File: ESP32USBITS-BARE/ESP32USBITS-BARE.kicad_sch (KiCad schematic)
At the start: 45 parts, among them IC2 74LVC, IC3 5PB1102, IC4 USBLC6, IC5 ESP32-S3-WROOM-1U-N16R8, IC6 RESET, IC7 BOOT, J1 I2S OUT, J2 Conn_01x10_Socket, J3 POWER IN, J4 USB-B CONNECTOR, U1 LD1117, Y2 22.5792MHz, Y3 24.5760Mhz

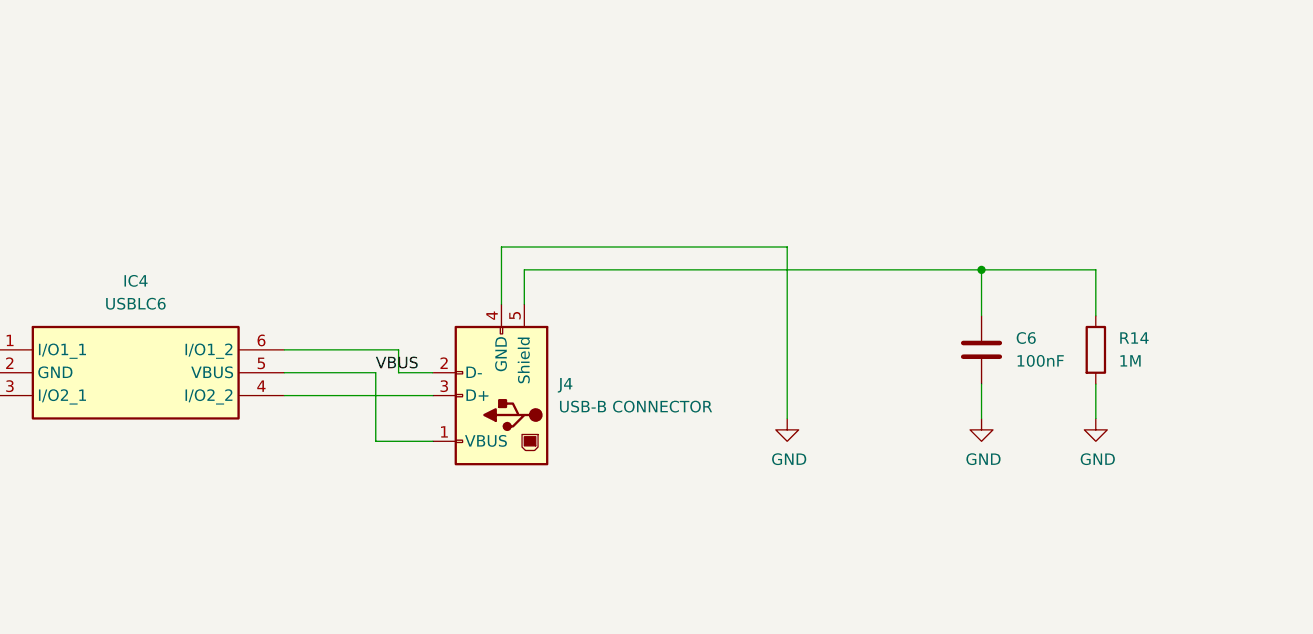
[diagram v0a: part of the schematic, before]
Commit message: more work
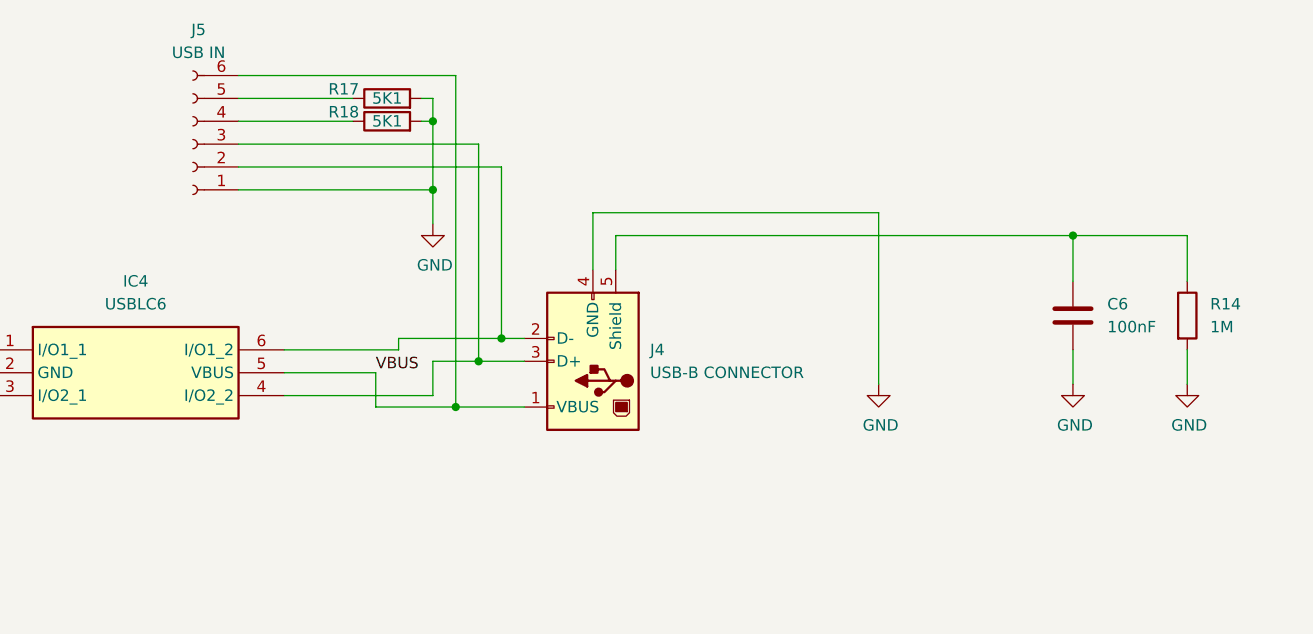
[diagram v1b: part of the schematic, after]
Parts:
- added J5: USB IN, Connector_Molex:Molex_KK-254_AE-6410-06A_1x06_P2.54mm_Vertical, symbol Connector:Conn_01x06_Socket
- added R17, R18: 5K1, Resistor_SMD:R_0805_2012Metric_Pad1.20x1.40mm_HandSolder, symbol Device:R
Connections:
- net GND: now also J5.1 (Pin_1), R17.2, R18.2
- net VBUS: now also J5.6 (Pin_6)
- net at IC4.6 (I/O1_2), J4.2 (D-): now also J5.2 (Pin_2)
- net at IC4.4 (I/O2_2), J4.3 (D+): now also J5.3 (Pin_3)
- new net: J5.4 (Pin_4), R18.1
- new net: J5.5 (Pin_5), R17.1
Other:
- moved on the sheet: C6, J4, R14
